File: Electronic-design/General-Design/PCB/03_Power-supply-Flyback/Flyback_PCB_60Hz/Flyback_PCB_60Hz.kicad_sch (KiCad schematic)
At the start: 58 parts, among them IC4 DPC817L-A-TR, IC5 UCC38C43DR, IC6 TL431ACLPR, J1 4300.0104, J6 Conn_01x02, Q1 NMOS, Q2 PNP, Q3 NPN, T3 750811351

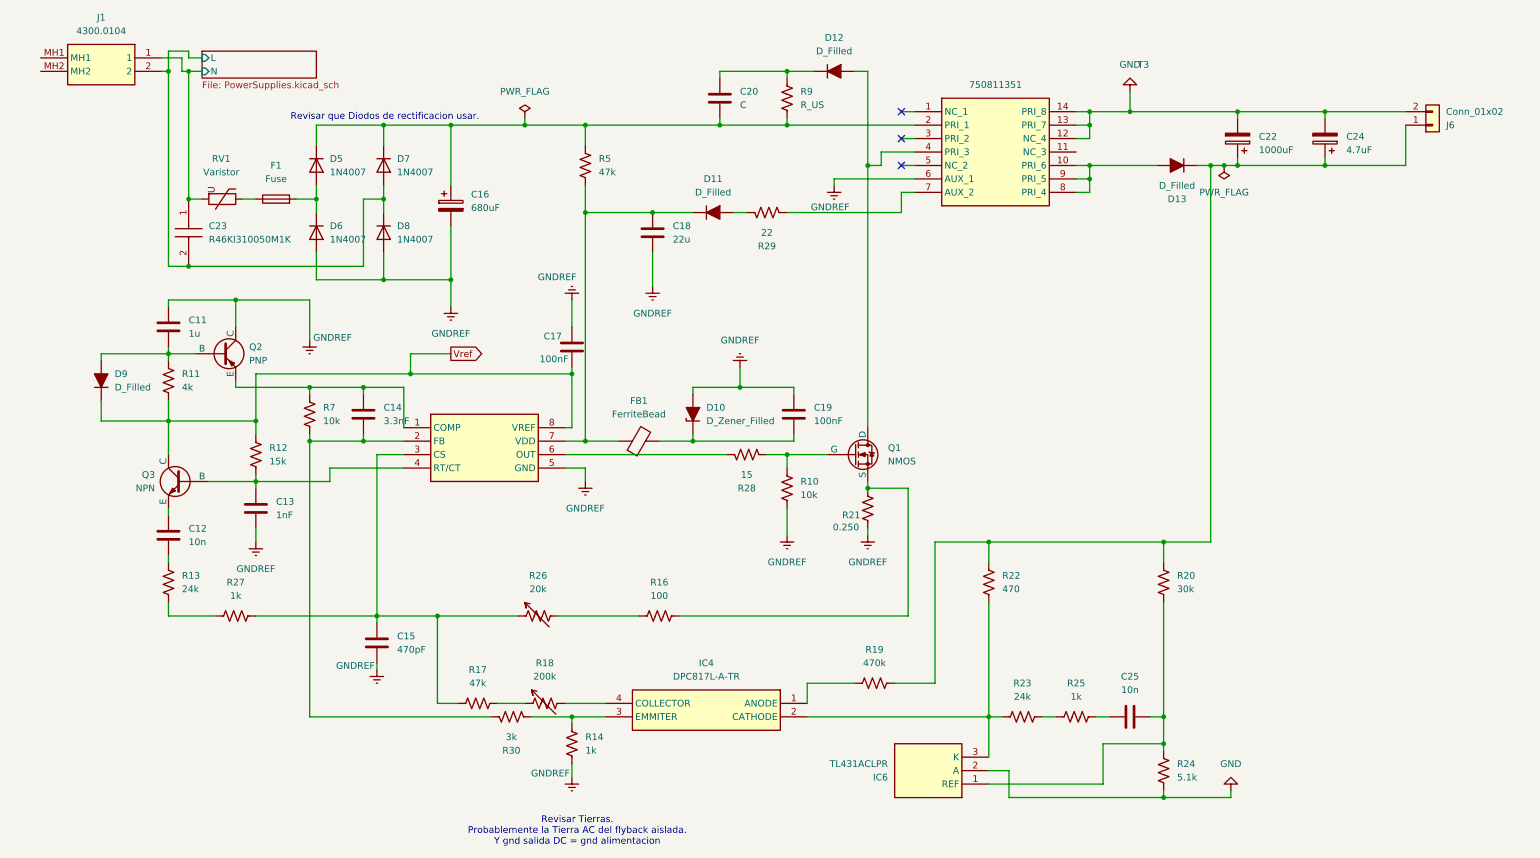
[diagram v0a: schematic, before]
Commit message: Flyback-Routing1
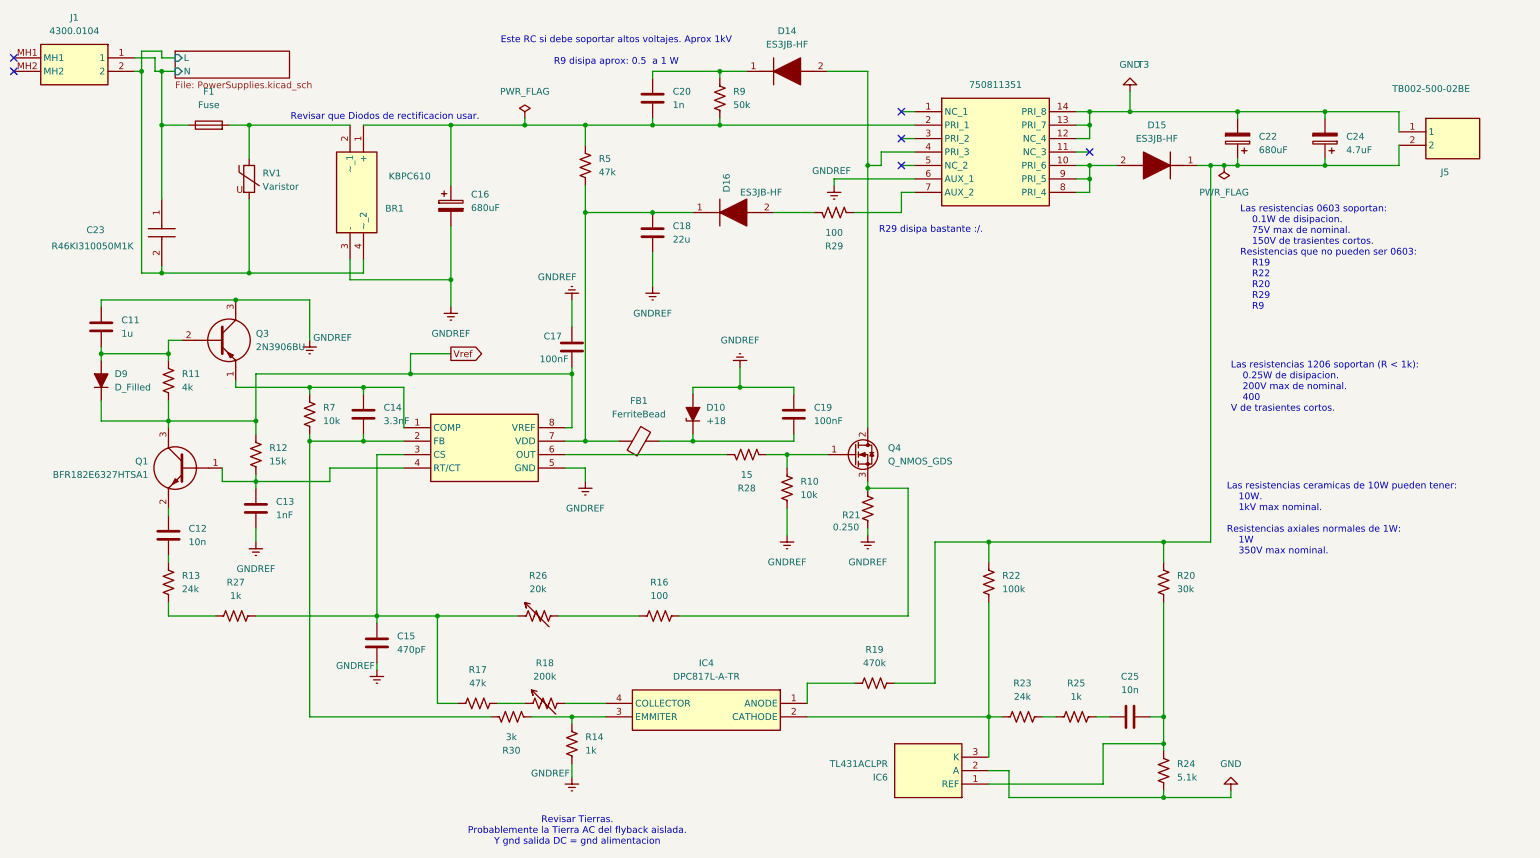
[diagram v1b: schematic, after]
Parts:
- removed D11, D12, D13: D_Filled, symbol Device:D_Filled
- removed D5, D6, D7, D8: 1N4007, Diode_THT:D_DO-41_SOD81_P10.16mm_Horizontal, symbol Diode:1N4007
- removed J6: Conn_01x02, Connector_JST:JST_XH_B2B-XH-A_1x02_P2.50mm_Vertical, symbol Connector_Generic:Conn_01x02
- removed Q1: NMOS, symbol Simulation_SPICE:NMOS
- removed Q2: PNP, symbol Simulation_SPICE:PNP
- removed Q3: NPN, symbol Simulation_SPICE:NPN
- added BR1: KBPC610, Flyback:KBPC610, symbol F_1_KBPC610:KBPC610
- added D14, D15, D16: ES3JB-HF, Flyback:DIOM5235X244N, symbol F_1_ES3JB-HF:ES3JB-HF
- added J5: TB002-500-02BE, Flyback:TB002-500-02BE, symbol F_1_TB002-500-02BE:TB002-500-02BE
- added Q1: BFR182E6327HTSA1, Flyback:NPN_SOT95P240X110-3N, symbol F_1_BFR182E6327HTSA1:BFR182E6327HTSA1
- added Q3: 2N3906BU, Flyback:2N3906BU, symbol F_1_2N3906BU:2N3906BU
- added Q4: Q_NMOS_GDS, Package_TO_SOT_THT:TO-220F-3_Vertical, symbol Transistor_FET:Q_NMOS_GDS
- C20: value C -> 1n; footprint (none) -> Capacitor_THT:C_Disc_D7.5mm_W4.4mm_P5.00mm
- C22: value 1000uF -> 680uF
- D10: value D_Zener_Filled -> +18; footprint (none) -> Diode_THT:D_DO-41_SOD81_P10.16mm_Horizontal
- D9: footprint (none) -> Diode_SMD:D_SMA_Handsoldering
- R19, R24: footprint Resistor_SMD:R_0603_1608Metric_Pad0.98x0.95mm_HandSolder -> Resistor_SMD:R_1206_3216Metric_Pad1.30x1.75mm_HandSolder
- R20: footprint Resistor_SMD:R_0603_1608Metric_Pad0.98x0.95mm_HandSolder -> Resistor_THT:R_Axial_DIN0414_L11.9mm_D4.5mm_P15.24mm_Horizontal
- R22: value 470 -> 100k; footprint Resistor_SMD:R_1206_3216Metric_Pad1.30x1.75mm_HandSolder -> Resistor_THT:R_Axial_DIN0414_L11.9mm_D4.5mm_P15.24mm_Horizontal
- R29: value 22 -> 100; footprint Resistor_SMD:R_1206_3216Metric_Pad1.30x1.75mm_HandSolder -> Resistor_THT:R_Axial_DIN0414_L11.9mm_D4.5mm_P15.24mm_Horizontal
- R9: value R_US -> 50k; footprint (none) -> Resistor_THT:R_Axial_Power_L50.0mm_W9.0mm_P60.96mm
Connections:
- net GND: now also J5.1
- net GNDREF: now also BR1.3 (-), Q3.3 (C)
- net Supplies/L: now also RV1.2, BR1.4 (~_2)
- net Supplies/N: now also F1.1; no longer RV1.2
- net Vref: now also Q1.3 (C)
- net at T3.10 (PRI_6), T3.8 (PRI_4), T3.9 (PRI_5): now also D15.2 (A)
- net at C16.1, C20.2, R5.1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: now also BR1.1 (+)
- net at T3.4 (PRI_3): now also D14.2 (A), Q4.2 (D)
- net at C22.1, C24.1, R19.1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: now also D15.1 (K), J5.2
- net at C11.2, D9.2 (A), R11.1: now also Q3.2 (B)
- net at C14.1, IC5.1 (COMP), R7.1: now also Q3.1 (E)
- net at F1.2: now also RV1.1, BR1.2 (~_1)
- net at C20.1, R9.1: now also D14.1 (K)
- net at C13.1, IC5.4 (RT/CT), R12.2: now also Q1.1 (B)
- net at C18.1, FB1.1, IC5.7 (VDD)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: now also D16.1 (K)
- net at C12.1: now also Q1.2 (E)
- net at R10.1, R28.2: now also Q4.1 (G)
- net at R29.1: now also D16.2 (A)
- net at R16.2, R21.1: now also Q4.3 (S)
- no-connect marks 3 -> 6
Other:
- note added: "Este RC si debe soportar altos voltajes. Aprox 1kV R9 disipa aprox: 0.5 a 1 W"
- note added: "Las resistencias 0603 soportan: 0.1W de disipacion. 75V max de nominal. 150V de trasientes cortos. Resistencias que no pueden ser 0603: R19 R22 R20 R29 R9"
- note added: "Las resistencias 1206 soportan (R < 1k): 0.25W de disipacion. 200V max de nominal. 400 V de trasientes cortos."
- note added: "Las resistencias ceramicas de 10W pueden tener: 10W. 1kV max nominal. Resistencias axiales normales de 1W: 1W 350V max nominal."
- note added: "R29 disipa bastante :/."
- moved on the sheet: C11, C20, C23, F1, J1, R29, R9, RV1

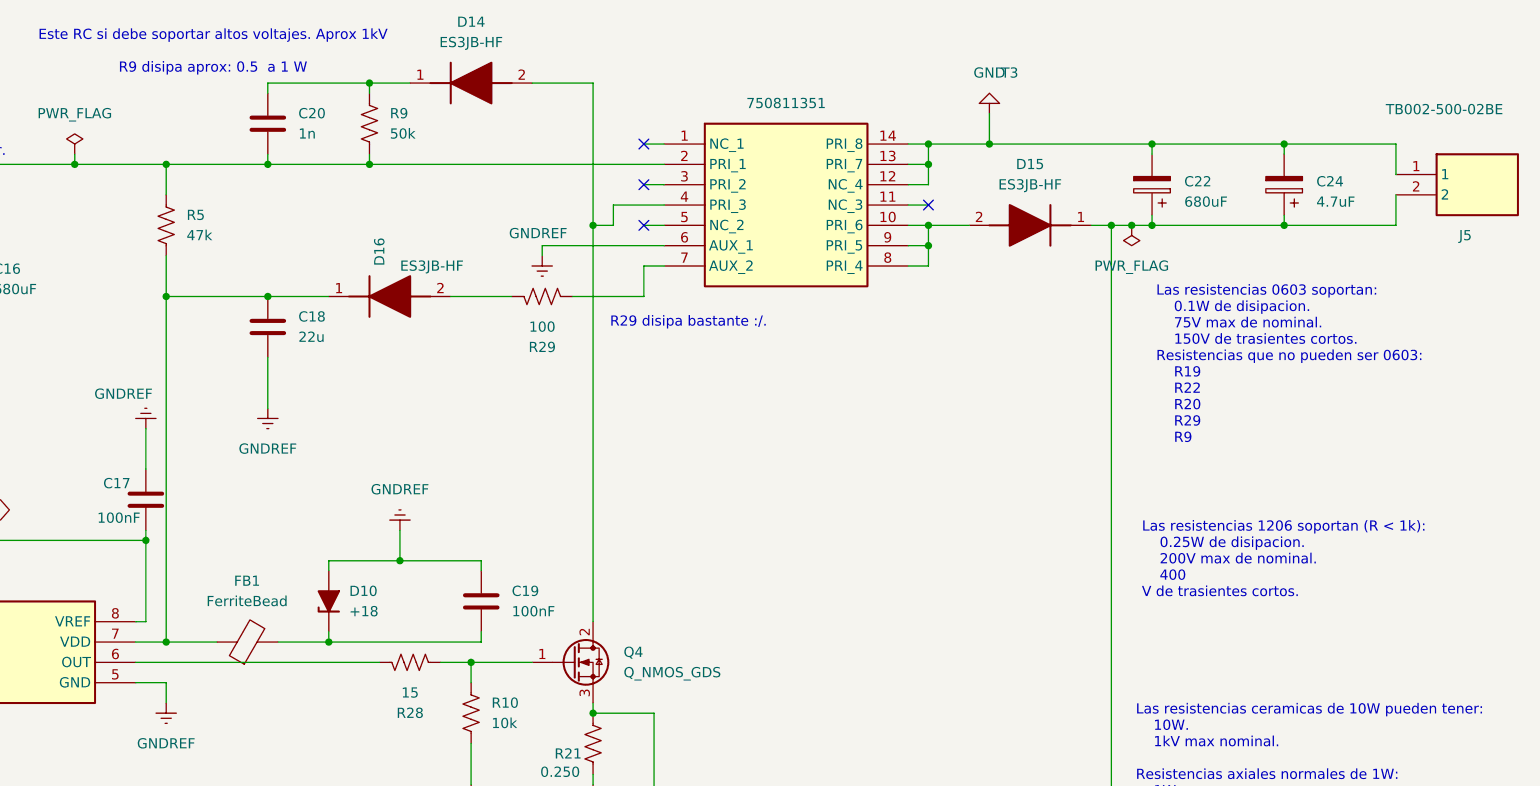
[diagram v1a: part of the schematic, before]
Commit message: Flyback-PCB-Final1
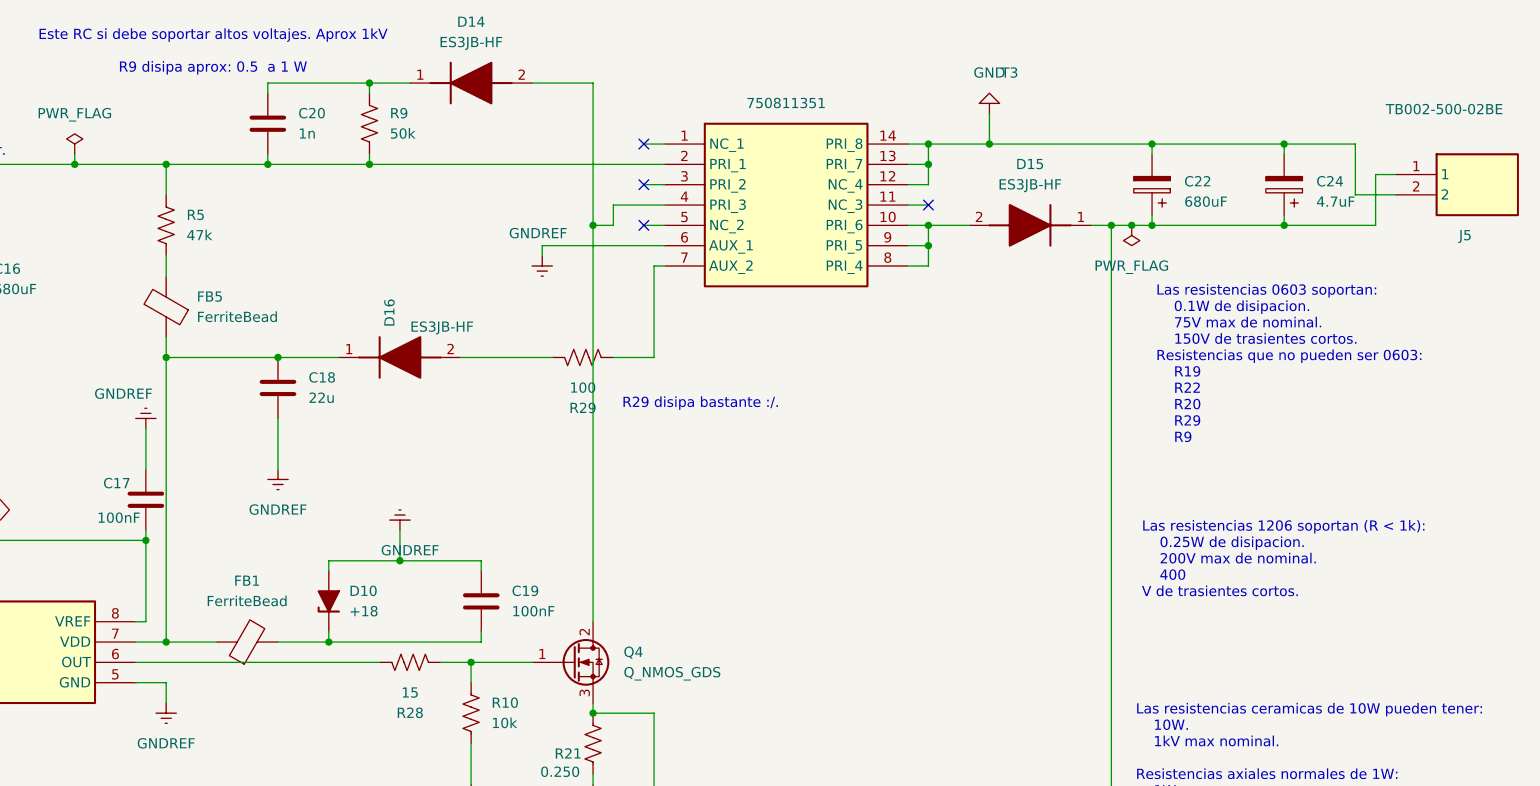
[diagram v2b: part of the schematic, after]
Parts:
- added FB5: FerriteBead, Flyback:BEADC1608X95N, symbol Device:FerriteBead
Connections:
- net GND: now also J5.2; no longer J5.1
- net at C22.1, C24.1, D15.1 (K)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: now also J5.1; no longer J5.2
- net at C18.1, D16.1 (K), FB1.1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: now also FB5.1; no longer R5.2
- new net: FB5.2, R5.2
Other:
- moved on the sheet: C18, D16, R29
